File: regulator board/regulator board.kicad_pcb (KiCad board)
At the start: 2 copper layers, 165 x 140 mm, 87 parts, among them J1 Phoenix connector 01x04, J2 C14 socket https://bit.ly/2kj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, J3 Pin socket, J4 Phoenix connector 01x04, J5 Phoenix connector 01x04, J6 Screw rerminal 01x03, J7 Phoenix connector 01x04, J8 Screw terminal 01x02, J9 Screw terminal 01x10, SW1 SW_Push_Dual, SW2 SW_Push_Dual, SW3 SW_Push_Dual, SW4 SW_Push_Dual, SW5 SW_Push_Dual, SW6 SW_Push_Dual, U1 MOC3063M, U10 MOC3063M, U11 PCF8574P https://bit.ly/2mbAL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, U12 PCF8574P https://bit.ly/2mbAL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, U2 PCF8574P https://bit.ly/2mbAL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, U3 MOC3063M, U4 MOC3063M, U5 MOC3063M, U6 MOC3063M, U7 ESP32-WROOM-32 https://bit.ly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, U8 MOC3063M, U9 MOC3063M

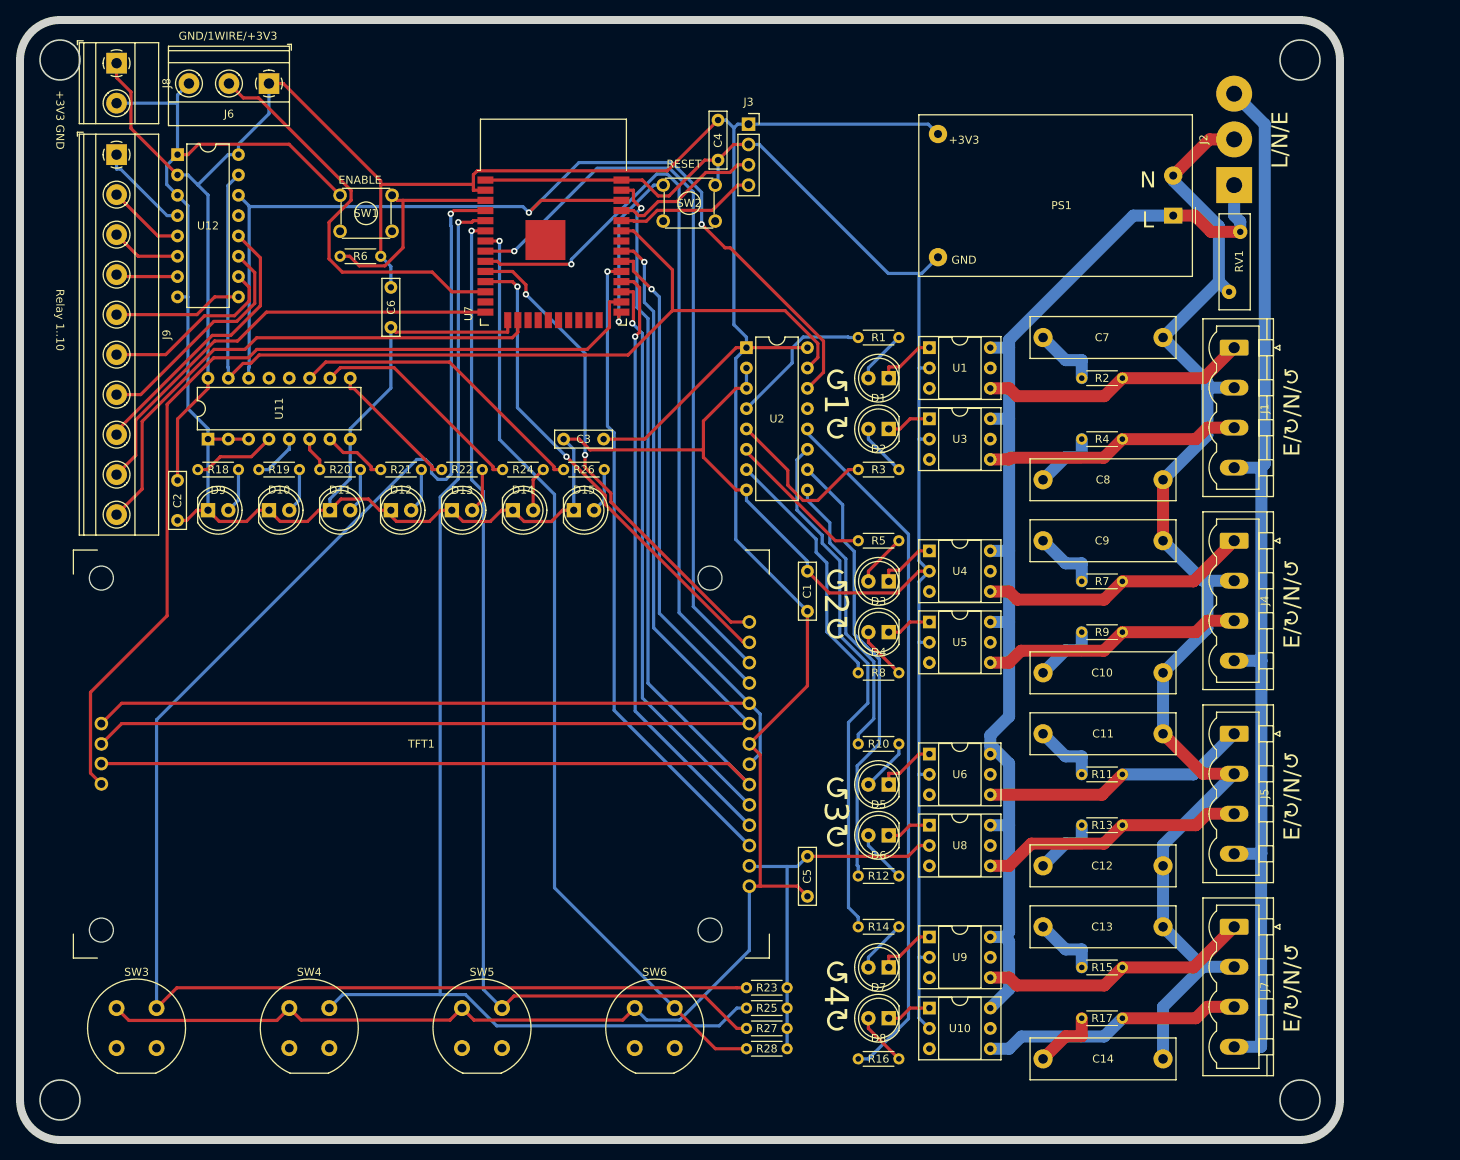
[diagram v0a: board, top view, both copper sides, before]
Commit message: Update PCB
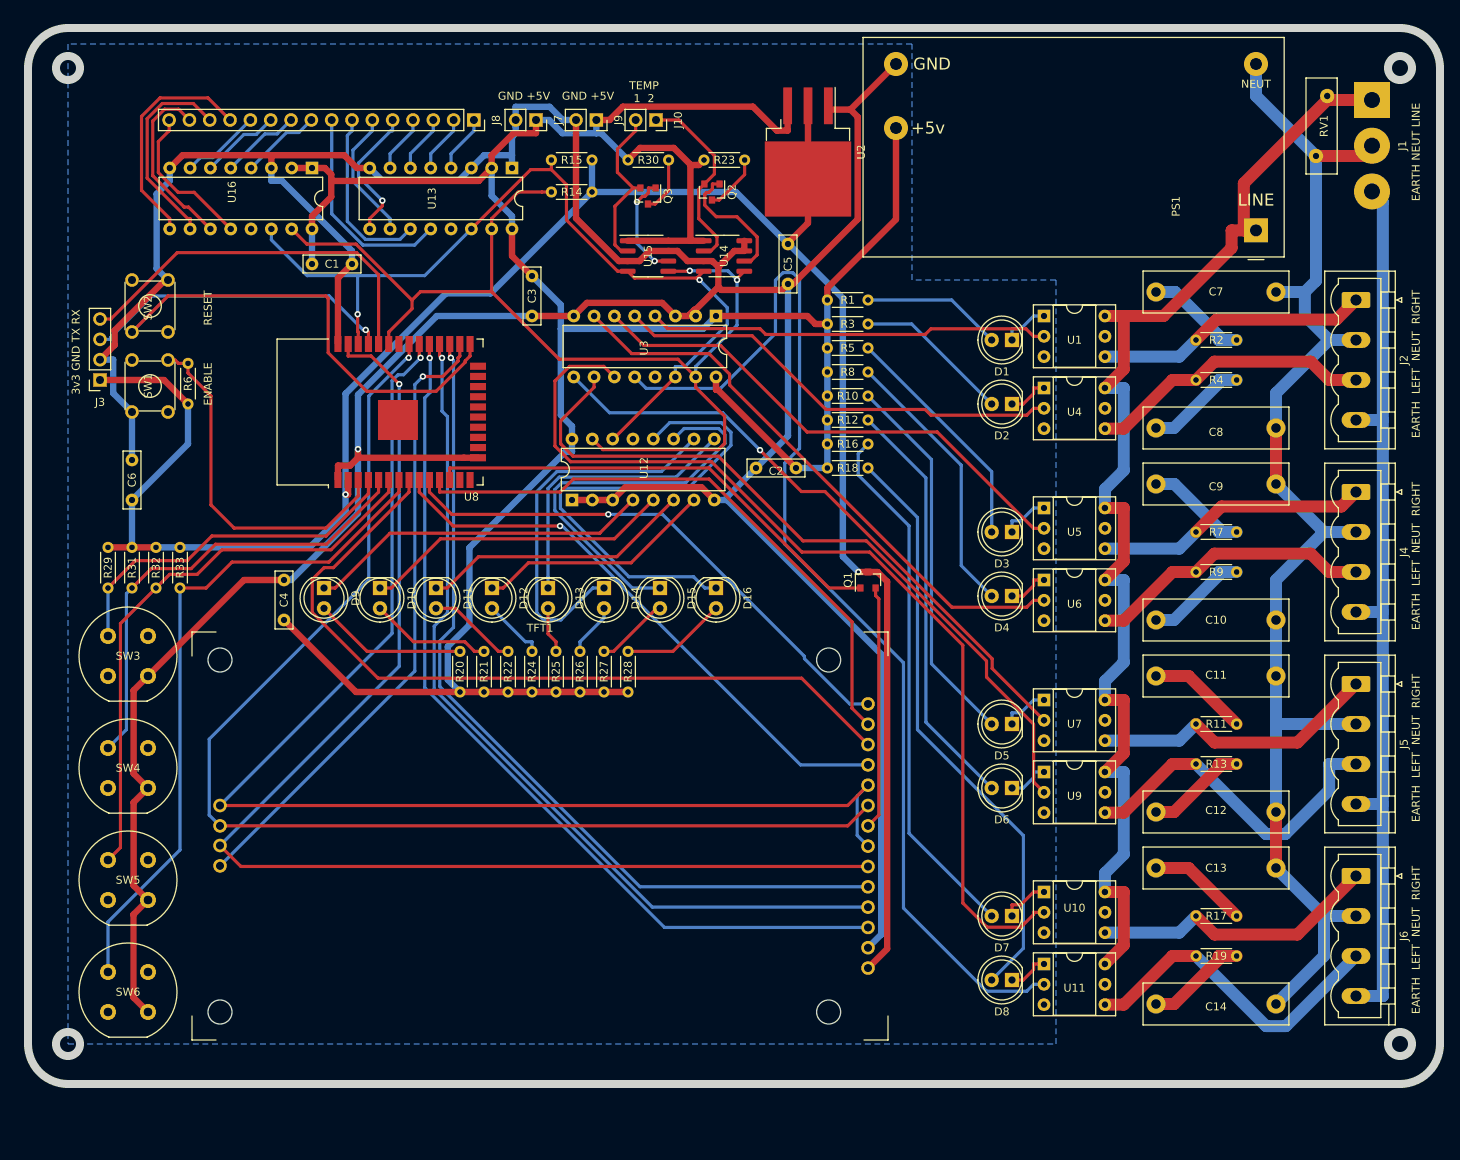
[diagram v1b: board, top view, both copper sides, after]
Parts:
- added D16: LED, LED_THT:LED_D5.0mm, F.Cu at (127.0, 91.0)
- added J10: Conn_01x02_Female, Connector_PinSocket_2.54mm:PinSocket_1x02_P2.54mm_Vertical, F.Cu at (119.5, 32.5)
- added Q1: BSS84, Package_TO_SOT_SMD:SOT-23, F.Cu at (146.0, 90.0)
- added Q2: BSS84, Package_TO_SOT_SMD:SOT-23, F.Cu at (126.5, 41.5)
- added Q3: BSS84, Package_TO_SOT_SMD:SOT-23, F.Cu at (118.5, 42.0)
- added R29: 10K, Resistor_THT:R_Axial_DIN0204_L3.6mm_D1.6mm_P5.08mm_Horizontal, F.Cu at (51.0, 91.0)
- added R30: 100, Resistor_THT:R_Axial_DIN0204_L3.6mm_D1.6mm_P5.08mm_Horizontal, F.Cu at (116.0, 37.5)
- added R31: 10K, Resistor_THT:R_Axial_DIN0204_L3.6mm_D1.6mm_P5.08mm_Horizontal, F.Cu at (54.0, 91.0)
- added R32: 10K, Resistor_THT:R_Axial_DIN0204_L3.6mm_D1.6mm_P5.08mm_Horizontal, F.Cu at (57.0, 91.0)
- added R33: 10K, Resistor_THT:R_Axial_DIN0204_L3.6mm_D1.6mm_P5.08mm_Horizontal, F.Cu at (60.0, 91.0)
- added U13: PCF8574P https://bit.ly/2mbALiV, Package_DIP:DIP-16_W7.62mm, F.Cu at (101.5, 38.5)
- added U14: DS2482S-100, Package_SO:SOP-8_3.76x4.96mm_P1.27mm, F.Cu at (128.0, 49.5)
- added U15: DS2482S-100, Package_SO:SOP-8_3.76x4.96mm_P1.27mm, F.Cu at (118.5, 49.5)
- added U16: PCF8574P https://bit.ly/2mbALiV, Package_DIP:DIP-16_W7.62mm, F.Cu at (76.5, 38.5)
- J1: value Phoenix connector 01x04 -> C14 socket https://bit.ly/2kjjjZt; footprint Connector_Phoenix_MSTB:PhoenixContact_MSTBVA_2,5_4-G_1x04_P5.00mm_Vertical -> Connector_Wire:SolderWirePad_1x03_P5.715mm_Drill2mm
- J2: value C14 socket https://bit.ly/2kjjjZt -> Phoenix connector 01x04; footprint Connector_Wire:SolderWirePad_1x03_P5.715mm_Drill2mm -> Connector_Phoenix_MSTB:PhoenixContact_MSTBVA_2,5_4-G_1x04_P5.00mm_Vertical
- J6: value Screw rerminal 01x03 -> Phoenix connector 01x04; footprint TerminalBlock_Phoenix:TerminalBlock_Phoenix_MKDS-1,5-3_1x03_P5.00mm_Horizontal -> Connector_Phoenix_MSTB:PhoenixContact_MSTBVA_2,5_4-G_1x04_P5.00mm_Vertical
- J7: value Phoenix connector 01x04 -> Conn_01x02_Female; footprint Connector_Phoenix_MSTB:PhoenixContact_MSTBVA_2,5_4-G_1x04_P5.00mm_Vertical -> Connector_PinSocket_2.54mm:PinSocket_1x02_P2.54mm_Vertical
- J8: value Screw terminal 01x02 -> Conn_01x16_Female; footprint TerminalBlock_Phoenix:TerminalBlock_Phoenix_MKDS-1,5-2_1x02_P5.00mm_Horizontal -> Connector_PinSocket_2.54mm:PinSocket_1x16_P2.54mm_Vertical
- J9: value Screw terminal 01x10 -> Conn_01x02_Female; footprint TerminalBlock_Phoenix:TerminalBlock_Phoenix_MKDS-1,5-10_1x10_P5.00mm_Horizontal -> Connector_PinSocket_2.54mm:PinSocket_1x02_P2.54mm_Vertical
- PS1: value SM-PLG06A-03 https://bit.ly/2kLhHrp -> Power supply https://bit.ly/2kBfKOu; footprint Converter_ACDC:Converter_ACDC_HiLink_HLK-PMxx -> Converter_ACDC:Converter_ACDC_MeanWell_IRM-20-xx_THT
- R14: value 330 -> 4k7
- R15: value 39 -> 4k7
- R18: value 180 -> 330
- R19: value 180 -> 39
- R23: value 10K -> 100
- R25, R27, R28: value 10K -> 180
- U11: value PCF8574P https://bit.ly/2mbALiV -> MOC3063M; footprint Package_DIP:DIP-16_W7.62mm -> Package_DIP:DIP-6_W7.62mm_Socket
- U2: value PCF8574P https://bit.ly/2mbALiV -> LM1117SX-3.3; footprint Package_DIP:DIP-16_W7.62mm -> Package_TO_SOT_SMD:TO-263-3_TabPin2
- U3: value MOC3063M -> PCF8574P https://bit.ly/2mbALiV; footprint Package_DIP:DIP-6_W7.62mm_Socket -> Package_DIP:DIP-16_W7.62mm
- U7: value ESP32-WROOM-32 https://bit.ly/2kIsByf -> MOC3063M; footprint RF_Module:ESP32-WROOM-32 -> Package_DIP:DIP-6_W7.62mm_Socket
- U8: value MOC3063M -> ESP-32S https://bit.ly/2kIsByf; footprint Package_DIP:DIP-6_W7.62mm_Socket -> RF_Module:ESP32-WROOM-32
- moved J6 168.2 mm to (207.0, 127.0), turned to 270 degrees
- moved J7 133.4 mm to (104.5, 32.5)
- moved R19 127.5 mm to (187.0, 137.0), turned to 0 degrees
- moved U11 123.4 mm to (168.0, 138.0), turned to 0 degrees
- moved R15 120.8 mm to (111.5, 37.5)
- moved R23 104.0 mm to (125.5, 37.5), turned to 0 degrees
- moved R14 99.5 mm to (111.5, 41.5)
- moved J3 87.1 mm to (50.0, 65.0), turned to 180 degrees
- moved U8 83.5 mm to (88.0, 69.0), turned to 90 degrees
- moved U7 83.5 mm to (168.0, 105.0)
- moved C4 82.8 mm to (73.0, 95.0), turned to 90 degrees
- moved C5 81.6 mm to (136.0, 48.0), turned to 270 degrees
- moved R18 78.7 mm to (146.0, 76.0)
- moved C2 77.3 mm to (137.0, 76.0), turned to 180 degrees
- moved R16 77.0 mm to (146.0, 73.0)
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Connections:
- C1 pad 1: +3V3 -> +5V
- C2 pad 1: +3V3 -> +5V
- C3 pad 1: +3V3 -> +5V
- C4 pad 1: +3V3 -> +5V
- D10 pad 1: GND -> Net-(D10-Pad1)
- D11 pad 1: GND -> Net-(D11-Pad1)
- D12 pad 1: GND -> Net-(D12-Pad1)
- D13 pad 1: GND -> Net-(D13-Pad1)
- D14 pad 1: GND -> Net-(D14-Pad1)
- D15 pad 1: GND -> Net-(D15-Pad1)
- D9 pad 1: GND -> Net-(D9-Pad1)
- J1 pad 1: Net-(J1-Pad1) -> LINE
- J1 pad 3: Net-(J1-Pad3) -> GNDPWR
- J2 pad 1: LINE -> Net-(J2-Pad1)
- J2 pad 3: GNDPWR -> Net-(J2-Pad3)
- J6 pad 1: +3V3 -> Net-(J6-Pad1)
- J6 pad 2: /1WIRE -> NEUT
- J6 pad 3: GND -> Net-(J6-Pad3)
- J7 pad 1: Net-(J7-Pad1) -> +5V
- J7 pad 2: NEUT -> GND
- J8 pad 1: +3V3 -> /R1
- J8 pad 2: GND -> /R2
- J9 pad 1: /R1 -> +5V
- J9 pad 2: /R2 -> GND
- PS1 pad 4: +3V3 -> +5V
- R1 pad 2: /P1 -> +5V
- R10 pad 2: /P5 -> +5V
- R12 pad 2: /P6 -> +5V
- R14 pad 1: Net-(D7-Pad2) -> +3V3
- R14 pad 2: /P7 -> SDA
- R15 pad 1: Net-(J7-Pad1) -> +3V3
- R15 pad 2: Net-(C13-Pad2) -> SCL
- R16 pad 1: Net-(D8-Pad2) -> Net-(D7-Pad2)
- R16 pad 2: /P8 -> +5V
- R17 pad 1: Net-(J7-Pad3) -> Net-(J6-Pad1)
- R17 pad 2: Net-(C14-Pad2) -> Net-(C13-Pad2)
- R18 pad 1: Net-(D9-Pad2) -> Net-(D8-Pad2)
- R18 pad 2: /L1 -> +5V
- R19 pad 1: Net-(D10-Pad2) -> Net-(J6-Pad3)
- R19 pad 2: /L2 -> Net-(C14-Pad2)
- R2 pad 1: Net-(J1-Pad1) -> Net-(J2-Pad1)
- R20 pad 1: Net-(D11-Pad2) -> +5V
- R20 pad 2: /L3 -> Net-(D9-Pad2)
- R21 pad 1: Net-(D12-Pad2) -> +5V
- R21 pad 2: /L4 -> Net-(D10-Pad2)
- R22 pad 1: Net-(D13-Pad2) -> +5V
- R22 pad 2: /L5 -> Net-(D11-Pad2)
- R23 pad 1: GND -> +5V
- R23 pad 2: /K1 -> Net-(Q2-Pad3)
- R24 pad 1: Net-(D14-Pad2) -> +5V
- R24 pad 2: /L6 -> Net-(D12-Pad2)
- R25 pad 1: GND -> +5V
- R25 pad 2: /K2 -> Net-(D13-Pad2)
- R26 pad 1: Net-(D15-Pad2) -> +5V
- R26 pad 2: /L7 -> Net-(D14-Pad2)
- R27 pad 1: GND -> +5V
- R27 pad 2: /K3 -> Net-(D15-Pad2)
- R28 pad 1: GND -> +5V
- R28 pad 2: /K4 -> Net-(D16-Pad2)
- R3 pad 2: /P2 -> +5V
- R4 pad 1: Net-(J1-Pad3) -> Net-(J2-Pad3)
- R5 pad 2: /P3 -> +5V
- R8 pad 2: /P4 -> +5V
- SW1 pad 2: /EN -> Net-(SW1-Pad2)
- SW1 pad 4: Net-(SW1-Pad4) -> /EN
- SW2 pad 2: GND -> Net-(SW2-Pad2)
- SW2 pad 4: Net-(SW2-Pad4) -> GND
- SW3 pad 1: +3V3 -> /K1
- SW3 pad 2: /K1 -> Net-(SW3-Pad2)
- SW3 pad 4: Net-(SW3-Pad4) -> GND
- SW4 pad 1: +3V3 -> /K2
- SW4 pad 2: /K2 -> Net-(SW4-Pad2)
- SW4 pad 4: Net-(SW4-Pad4) -> GND
- SW5 pad 1: +3V3 -> /K3
- SW5 pad 2: /K3 -> Net-(SW5-Pad2)
- SW5 pad 4: Net-(SW5-Pad4) -> GND
- SW6 pad 1: +3V3 -> /K4
- SW6 pad 2: /K4 -> Net-(SW6-Pad2)
- SW6 pad 4: Net-(SW6-Pad4) -> GND
- TFT1 pad 7: +3V3 -> Net-(Q1-Pad2)
- U1 pad 2: GND -> /P1
- U1 pad 4: Net-(J1-Pad1) -> Net-(J2-Pad1)
- U10 pad 1: Net-(D8-Pad1) -> Net-(D7-Pad1)
- U10 pad 2: GND -> /P7
- U10 pad 4: Net-(J7-Pad3) -> Net-(J6-Pad1)
- U11 pad 1: GND -> Net-(D8-Pad1)
- U11 pad 2: GND -> /P8
- U11 pad 3: GND -> Net-(U11-Pad3)
- U11 pad 4: /L1 -> Net-(J6-Pad3)
- U11 pad 5: /L2 -> Net-(U11-Pad5)
- U11 pad 6: /L3 -> LINE
- U12 pad 10: /R6 -> Net-(D14-Pad1)
- U12 pad 11: /R7 -> Net-(D15-Pad1)
- U12 pad 12: /R8 -> Net-(D16-Pad1)
- U12 pad 16: +3V3 -> +5V
- U12 pad 2: +3V3 -> GND
- U12 pad 4: /R1 -> Net-(D9-Pad1)
- U12 pad 5: /R2 -> Net-(D10-Pad1)
- U12 pad 6: /R3 -> Net-(D11-Pad1)
- U12 pad 7: /R4 -> Net-(D12-Pad1)
- U12 pad 9: /R5 -> Net-(D13-Pad1)
- U2 pad 1: +3V3 -> GND
- U2 pad 2: GND -> +3V3
- U2 pad 3: GND -> +5V
- U3 pad 1: Net-(D2-Pad1) -> +5V
- U3 pad 3: Net-(U3-Pad3) -> GND
- U3 pad 4: Net-(J1-Pad3) -> /P1
- U3 pad 5: Net-(U3-Pad5) -> /P2
- U3 pad 6: LINE -> /P3
- U4 pad 1: Net-(D3-Pad1) -> Net-(D2-Pad1)
- U4 pad 2: GND -> /P2
- U4 pad 4: Net-(J4-Pad1) -> Net-(J2-Pad3)
- U5 pad 1: Net-(D4-Pad1) -> Net-(D3-Pad1)
- U5 pad 2: GND -> /P3
- U5 pad 4: Net-(J4-Pad3) -> Net-(J4-Pad1)
- U6 pad 1: Net-(D5-Pad1) -> Net-(D4-Pad1)
- U6 pad 2: GND -> /P4
- U6 pad 4: Net-(J5-Pad1) -> Net-(J4-Pad3)
- U7 pad 1: GND -> Net-(D5-Pad1)
- U7 pad 2: +3V3 -> /P5
- U7 pad 3: /EN -> Net-(U7-Pad3)
- U7 pad 4: /K1 -> Net-(J5-Pad1)
- U7 pad 5: /K2 -> Net-(U7-Pad5)
- U7 pad 6: /K3 -> LINE
- U8 pad 1: Net-(D6-Pad1) -> GND
- U8 pad 2: GND -> +3V3
- U8 pad 3: Net-(U8-Pad3) -> /EN
- U8 pad 4: Net-(J5-Pad3) -> /K1
- U8 pad 5: Net-(U8-Pad5) -> /K2
- U8 pad 6: LINE -> /K3
- U9 pad 1: Net-(D7-Pad1) -> Net-(D6-Pad1)
- U9 pad 2: GND -> /P6
- U9 pad 4: Net-(J7-Pad1) -> Net-(J5-Pad3)
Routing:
- net +5V: track 0.00 -> 346.5 mm
- net /K1: track 200.1 -> 45.1 mm, vias 1 -> 0
- net +3V3: track 422.6 -> 270.3 mm, vias 0 -> 2
- net /K2: track 156.3 -> 58.5 mm, vias 1 -> 0
- net Net-(D8-Pad2): track 6.66 -> 73.7 mm
- net Net-(D16-Pad1): track 0.00 -> 62.0 mm
- net /K3: track 133.3 -> 72.1 mm, vias 1 -> 0
- net Net-(D7-Pad2): track 6.66 -> 66.4 mm
- net /TFT_LED: track 0.00 -> 59.0 mm
- net /P7: track 65.4 -> 122.7 mm
- net /R10: track 66.1 -> 10.0 mm
- net /P8: track 87.3 -> 139.1 mm
- net Net-(D15-Pad1): track 0.00 -> 51.8 mm
- net /1WIRE: track 51.7 -> 0.00 mm
- net Net-(D14-Pad1): track 0.00 -> 47.9 mm
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- added copper zone on B.Cu, net GND
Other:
- board size 165 x 140 mm -> 176.5 x 132 mm
- net class LogicPower added: clearance 0.4, trace_width 0.8, via_dia 0.8, via_drill 0.4
- board text added: "+5v"
- board text added: "3v3 GND TX RX"
- board text added: "EARTH LEFT NEUT RIGHT"
- board text added: "EARTH NEUT LINE"
- board text added: "GND +5V"
- board text added: "LINE"
- board text added: "NEUT"
- board text added: "TEMP 1 2"
- board text removed: "+3V3"
- board text removed: "+3V3 GND"
- board text removed: "E/↻/N/↺"
- board text removed: "GND/1WIRE/+3V3"
- board text removed: "L"
- board text removed: "L/N/E"
- board text removed: "N"
- board text removed: "Relay 1..10"
- board text removed: "↺1↻"
- board text removed: "↺2↻"
- board text removed: "↺3↻"
- board text removed: "↺4↻"
